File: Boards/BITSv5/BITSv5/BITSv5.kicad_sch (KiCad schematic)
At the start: 87 parts, among them J1 Conn_01x10_Pin, J2 USB_C_Receptacle_USB2.0, J3 Conn_01x06, J4 Conn_01x02, Q1 Q_NMOS_GSD, Q2 Q_PMOS_GSD, SW2 PTM, SW3 SLIDE, U1 MCU_RaspberryPi_RP2040_RP2040, U10 USBLC6-2SC6, U2 W25Q128JVS, U3 MAX-M10S, U4 MAX77857, U5 TPS61232DRCR, U6 XBee_SMT, U7 TPS2121RUXR, U8 LT6703CDC-3, U9 TVS1800DRVR, Y1 12MHz

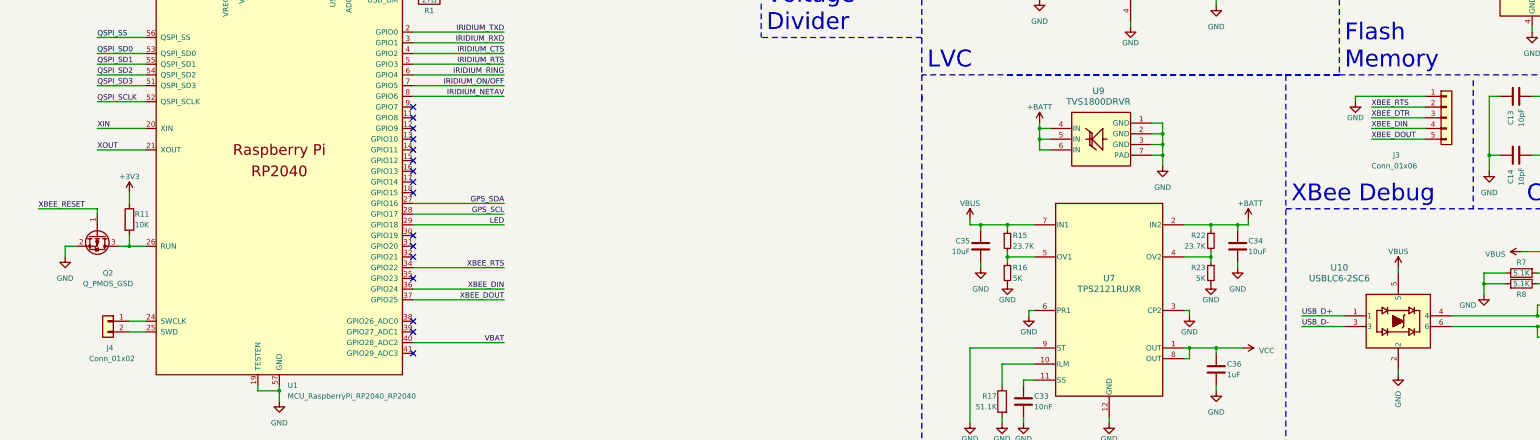
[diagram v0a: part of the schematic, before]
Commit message: several hundred bits v5 errors later
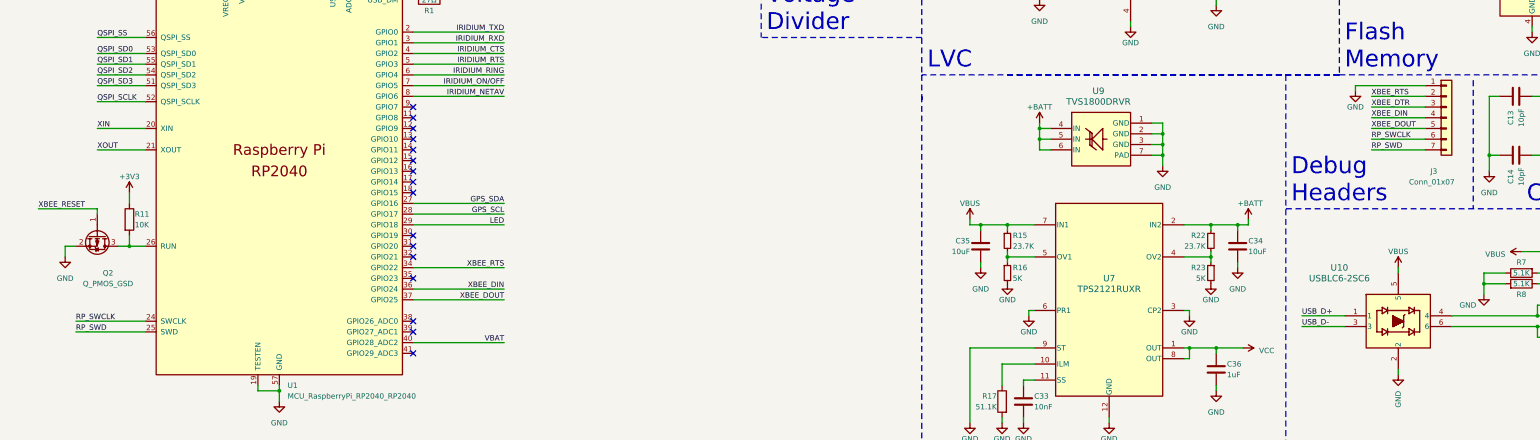
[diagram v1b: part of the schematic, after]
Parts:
- removed J4: Conn_01x02, symbol Connector_Generic:Conn_01x02
- BT1: footprint GHOULFootPrints:XT30PW-M -> BITSv5:XT30PW-M
- J3: value Conn_01x06 -> Conn_01x07; footprint Connector_JST:JST_EH_B5B-EH-A_1x05_P2.50mm_Vertical -> Connector_PinSocket_2.54mm:PinSocket_1x07_P2.54mm_Vertical; symbol Connector_Generic:Conn_01x05 -> Connector_Generic:Conn_01x07
- L2: footprint 1616_Inductor:IND_XAL4020_4X4_COC-M -> BITSv5:IND_XAL4020_4X4_COC-M
- U1: footprint RP2040_minimal:RP2040-QFN-56 -> BITSv5:RP2040-QFN-56
- U4: footprint MAX77857:MAX77857-35WLP -> BITSv5:MAX77857-35WLP
- U5: footprint TPS61232:DRC0010G -> BITSv5:TPS61232
- U8: footprint DFN-3_DC_LIT -> BITSv5:DFN-3_DC_LIT
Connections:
- net RP_SWCLK: now reaches U1.24 (SWCLK)
- net RP_SWCLK: now also J3.6 (Pin_6)
- net RP_SWD: now reaches U1.25 (SWD)
- net RP_SWD: now also J3.7 (Pin_7)
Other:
- note added: "Debug Headers"
- note removed: "XBee Debug"
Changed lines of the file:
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@@
     (stroke (width 0) (type default))
   )
-  (wire (pts (xy 336.55 74.93) (xy 349.25 74.93))
-    (stroke (width 0) (type default))
-  )
   (wire (pts (xy 287.02 81.28) (xy 287.02 78.74))
     (stroke (width 0) (type default))
@@
     (stroke (width 0) (type default))
   )
-  (wire (pts (xy 332.74 71.12) (xy 332.74 69.85))
+  (wire (pts (xy 332.74 68.58) (xy 332.74 67.31))
     (stroke (width 0) (type default))
   )
@@
     (stroke (width 0) (type default))
   )
-  (wire (pts (xy 336.55 77.47) (xy 349.25 77.47))
-    (stroke (width 0) (type default))
-  )
   (wire (pts (xy 29.21 219.71) (xy 29.21 220.98))
     (stroke (width 0) (type default))
@@
     (stroke (width 0) (type default))
   )
+  (wire (pts (xy 336.55 69.85) (xy 349.25 69.85))
+    (stroke (width 0) (type default))
+  )
   (wire (pts (xy 374.65 83.82) (xy 387.35 83.82))
     (stroke (width 0) (type default))
@@
     (stroke (width 0) (type default))
   )
-  (wire (pts (xy 332.74 69.85) (xy 349.25 69.85))
-    (stroke (width 0) (type default))
-  )
   (polyline (pts (xy 328.93 64.77) (xy 229.87 64.77))
     (stroke (width 0) (type dash_dot))
@@
     (stroke (width 0) (type dash_dot))
   )
+  (wire (pts (xy 336.55 72.39) (xy 349.25 72.39))
+    (stroke (width 0) (type default))
+  )
   (wire (pts (xy 93.98 21.59) (xy 93.98 36.83))
     (stroke (width 0) (type default))
@@
     (stroke (width 0) (type default))
   )
+  (wire (pts (xy 336.55 80.01) (xy 349.25 80.01))
+    (stroke (width 0) (type default))
+  )
   (wire (pts (xy 391.16 30.48) (xy 391.16 33.02))
     (stroke (width 0) (type default))
@@
     (stroke (width 0) (type default))
   )
-  (wire (pts (xy 336.55 80.01) (xy 349.25 80.01))
-    (stroke (width 0) (type default))
-  )
   (wire (pts (xy 86.36 36.83) (xy 86.36 21.59))
     (stroke (width 0) (type default))
@@
     (stroke (width 0) (type default))
   )
+  (wire (pts (xy 336.55 74.93) (xy 349.25 74.93))
+    (stroke (width 0) (type default))
+  )
   (wire (pts (xy 320.04 121.92) (xy 330.2 121.92))
     (stroke (width 0) (type default))
@@
     (stroke (width 0) (type default))
   )
+  (wire (pts (xy 336.55 82.55) (xy 349.25 82.55))
+    (stroke (width 0) (type default))
+  )
   (wire (pts (xy 285.75 250.19) (xy 285.75 252.73))
     (stroke (width 0) (type default))
@@
     (stroke (width 0) (type default))
   )
+  (wire (pts (xy 332.74 67.31) (xy 349.25 67.31))
+    (stroke (width 0) (type default))
+  )
   (wire (pts (xy 271.78 181.61) (xy 271.78 172.72))
     (stroke (width 0) (type default))
@@
     (stroke (width 0) (type default))
   )
-  (wire (pts (xy 336.55 72.39) (xy 349.25 72.39))
-    (stroke (width 0) (type default))
-  )
   (wire (pts (xy 59.69 21.59) (xy 57.15 21.59))
     (stroke (width 0) (type default))
@@
     (stroke (width 0) (type default))
   )
-  (wire (pts (xy 41.91 125.73) (xy 45.72 125.73))
+  (wire (pts (xy 29.21 125.73) (xy 45.72 125.73))
     (stroke (width 0) (type default))
   )
@@
     (stroke (width 0) (type default))
   )
+  (wire (pts (xy 336.55 77.47) (xy 349.25 77.47))
+    (stroke (width 0) (type default))
+  )
   (wire (pts (xy 119.38 210.82) (xy 119.38 212.09))
     (stroke (width 0) (type default))
@@
     (stroke (width 0) (type default))
   )
-  (wire (pts (xy 41.91 123.19) (xy 45.72 123.19))
+  (wire (pts (xy 29.21 123.19) (xy 45.72 123.19))
     (stroke (width 0) (type default))
   )
@@
     (effects (font (size 4 4)) (justify left bottom))
   )
-  (text "XBee Debug" (at 317.5 95.25 0)
+  (text "Debug\nHeaders" (at 317.5 95.25 0)
     (effects (font (size 4 4)) (justify left bottom))
   )
@@
     (effects (font (size 1.27 1.27)) (justify left bottom))
   )
-  (label "XBEE_DTR" (at 336.55 74.93 0) (fields_autoplaced)
+  (label "XBEE_DTR" (at 336.55 72.39 0) (fields_autoplaced)
     (effects (font (size 1.27 1.27)) (justify left bottom))
   )
@@
     (effects (font (size 1.27 1.27)) (justify left bottom))
   )
-  (label "XBEE_DOUT" (at 336.55 80.01 0) (fields_autoplaced)
+  (label "XBEE_DOUT" (at 336.55 77.47 0) (fields_autoplaced)
+    (effects (font (size 1.27 1.27)) (justify left bottom))
+  )
+  (label "RP_SWCLK" (at 336.55 80.01 0) (fields_autoplaced)
+    (effects (font (size 1.27 1.27)) (justify left bottom))
+  )
+  (label "RP_SWD" (at 336.55 82.55 0) (fields_autoplaced)
     (effects (font (size 1.27 1.27)) (justify left bottom))
   )
@@
     (effects (font (size 1.27 1.27)) (justify left bottom))
   )
-  (label "XBEE_RTS" (at 336.55 72.39 0) (fields_autoplaced)
+  (label "XBEE_RTS" (at 336.55 69.85 0) (fields_autoplaced)
     (effects (font (size 1.27 1.27)) (justify left bottom))
   )
@@
     (effects (font (size 1.27 1.27)) (justify left bottom))
   )
-  (label "XBEE_DIN" (at 336.55 77.47 0) (fields_autoplaced)
+  (label "XBEE_DIN" (at 336.55 74.93 0) (fields_autoplaced)
     (effects (font (size 1.27 1.27)) (justify left bottom))
   )
@@
     (effects (font (size 1.27 1.27)) (justify right bottom))
   )
+  (label "RP_SWCLK" (at 29.21 123.19 0) (fields_autoplaced)
+    (effects (font (size 1.27 1.27)) (justify left bottom))
+  )
   (label "XBEE_DOUT" (at 326.39 207.01 0) (fields_autoplaced)
     (effects (font (size 1.27 1.27)) (justify left bottom))
@@
     (effects (font (size 1.27 1.27)) (justify right bottom))
   )
+  (label "RP_SWD" (at 29.21 125.73 0) (fields_autoplaced)
+    (effects (font (size 1.27 1.27)) (justify left bottom))
+  )
   (label "QSPI_SD2" (at 353.06 43.18 0) (fields_autoplaced)
     (effects (font (size 1.27 1.27)) (justify left bottom))
@@
     )
   )
-  (symbol (lib_id "Connector_Generic:Conn_01x05") (at 354.33 74.93 0) (unit 1)
+  (symbol (lib_id "Connector_Generic:Conn_01x07") (at 354.33 74.93 0) (unit 1)
     (in_bom yes) (on_board yes) (dnp no)
-    (property "Reference" "J3" (at 341.63 83.82 0)
+    (property "Reference" "J3" (at 350.52 87.63 0)
       (effects (font (size 1.27 1.27)) (justify left))
     )
-    (property "Value" "Conn_01x06" (at 336.55 86.36 0)
+    (property "Value" "Conn_01x07" (at 345.44 90.17 0)
       (effects (font (size 1.27 1.27)) (justify left))
     )
-    (property "Footprint" "Connector_JST:JST_EH_B5B-EH-A_1x05_P2.50mm_Vertical" (at 354.33 74.93 0)
+    (property "Footprint" "Connector_PinSocket_2.54mm:PinSocket_1x07_P2.54mm_Vertical" (at 354.33 74.93 0)
       (effects (font (size 1.27 1.27)) hide)
     )
@@
     (pin "4")
     (pin "5")
+    (pin "6")
+    (pin "7")
     (instances
       (project "BITSv5"
@@
       (effects (font (size 1.27 1.27)))
     )
-    (property "Footprint" "1616_Inductor:IND_XAL4020_4X4_COC-M" (at 250.19 172.72 0)
+    (property "Footprint" "BITSv5:IND_XAL4020_4X4_COC-M" (at 250.19 172.72 0)
       (effects (font (size 1.27 1.27)) hide)
     )
@@
       (effects (font (size 1.27 1.27)) (justify left) hide)
     )
-    (property "Footprint" "GHOULFootPrints:XT30PW-M" (at 199.39 22.606 90)
+    (property "Footprint" "BITSv5:XT30PW-M" (at 199.39 22.606 90)
       (effects (font (size 1.27 1.27)) hide)
     )
@@
       (effects (font (size 1.524 1.524)))
     )
-    (property "Footprint" "DFN-3_DC_LIT" (at 260.35 25.4 0)
+    (property "Footprint" "BITSv5:DFN-3_DC_LIT" (at 260.35 25.4 0)
       (effects (font (size 1.27 1.27) italic) hide)
     )
@@
     )
   )
-  (symbol (lib_id "Connector_Generic:Conn_01x02") (at 36.83 123.19 0) (mirror y) (unit 1)
-    (in_bom yes) (on_board yes) (dnp no)
-    (property "Reference" "J4" (at 38.1 129.54 0)
-      (effects (font (size 1.27 1.27)) (justify left))
-    )
-    (property "Value" "Conn_01x02" (at 43.18 132.08 0)
-      (effects (font (size 1.27 1.27)) (justify left))
-    )
-    (property "Footprint" "" (at 36.83 123.19 0)
-      (effects (font (size 1.27 1.27)) hide)
-    )
-    (property "Datasheet" "~" (at 36.83 123.19 0)
-      (effects (font (size 1.27 1.27)) hide)
-    )
-    (pin "1")
-    (pin "2")
-    (instances
-      (project "BITSv5"
-        (path "/55a258d3-b7da-466a-a6cc-38d8142826fc"
-          (reference "J4") (unit 1)
-        )
-      )
-    )
-  )
   (symbol (lib_id "power:+5V") (at 302.26 186.69 0) (unit 1)
     (in_bom yes) (on_board yes) (dnp no) (fields_autoplaced)
@@
     )
   )
-  (symbol (lib_id "power:GND") (at 332.74 71.12 0) (unit 1)
+  (symbol (lib_id "power:GND") (at 332.74 68.58 0) (unit 1)
     (in_bom yes) (on_board yes) (dnp no)
-    (property "Reference" "#PWR062" (at 332.74 77.47 0)
+    (property "Reference" "#PWR062" (at 332.74 74.93 0)
       (effects (font (size 1.27 1.27)) hide)
     )
-    (property "Value" "GND" (at 332.74 74.93 0)
+    (property "Value" "GND" (at 332.74 72.39 0)
       (effects (font (size 1.27 1.27)))
     )
-    (property "Footprint" "" (at 332.74 71.12 0)
+    (property "Footprint" "" (at 332.74 68.58 0)
       (effects (font (size 1.27 1.27)) hide)
     )
-    (property "Datasheet" "" (at 332.74 71.12 0)
+    (property "Datasheet" "" (at 332.74 68.58 0)
       (effects (font (size 1.27 1.27)) hide)
     )
@@
       (effects (font (size 1.27 1.27)) (justify left))
     )
-    (property "Footprint" "RP2040_minimal:RP2040-QFN-56" (at 58.42 87.63 0)
+    (property "Footprint" "BITSv5:RP2040-QFN-56" (at 58.42 87.63 0)
       (effects (font (size 1.27 1.27)) hide)
     )
@@
       (effects (font (size 1.524 1.524)))
     )
-    (property "Footprint" "TPS61232:DRC0010G" (at 250.19 191.77 0)
+    (property "Footprint" "BITSv5:TPS61232" (at 250.19 191.77 0)
       (effects (font (size 1.27 1.27) italic) hide)
     )
@@
       (effects (font (size 1.524 1.524)))
     )
-    (property "Footprint" "MAX77857:MAX77857-35WLP" (at 39.37 201.93 0)
+    (property "Footprint" "BITSv5:MAX77857-35WLP" (at 39.37 201.93 0)
       (effects (font (size 1.27 1.27) italic) hide)
     )
